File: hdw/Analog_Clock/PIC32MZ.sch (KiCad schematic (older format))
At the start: 3 parts

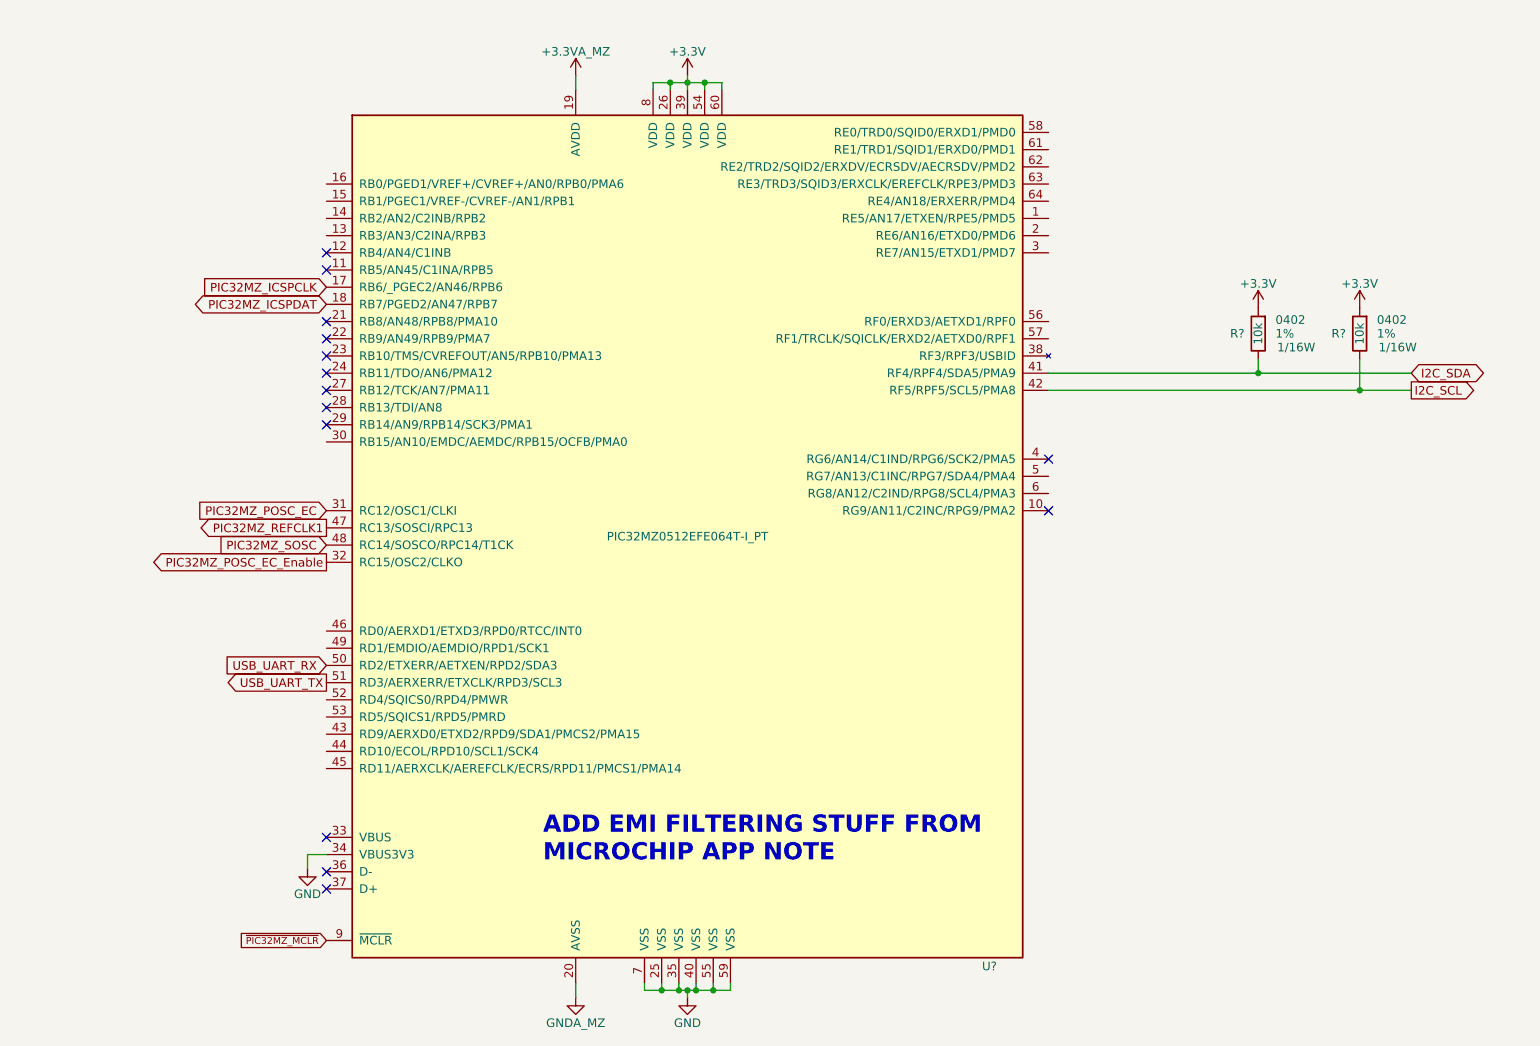
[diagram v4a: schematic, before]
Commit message: more analog work, added some more sch stuff
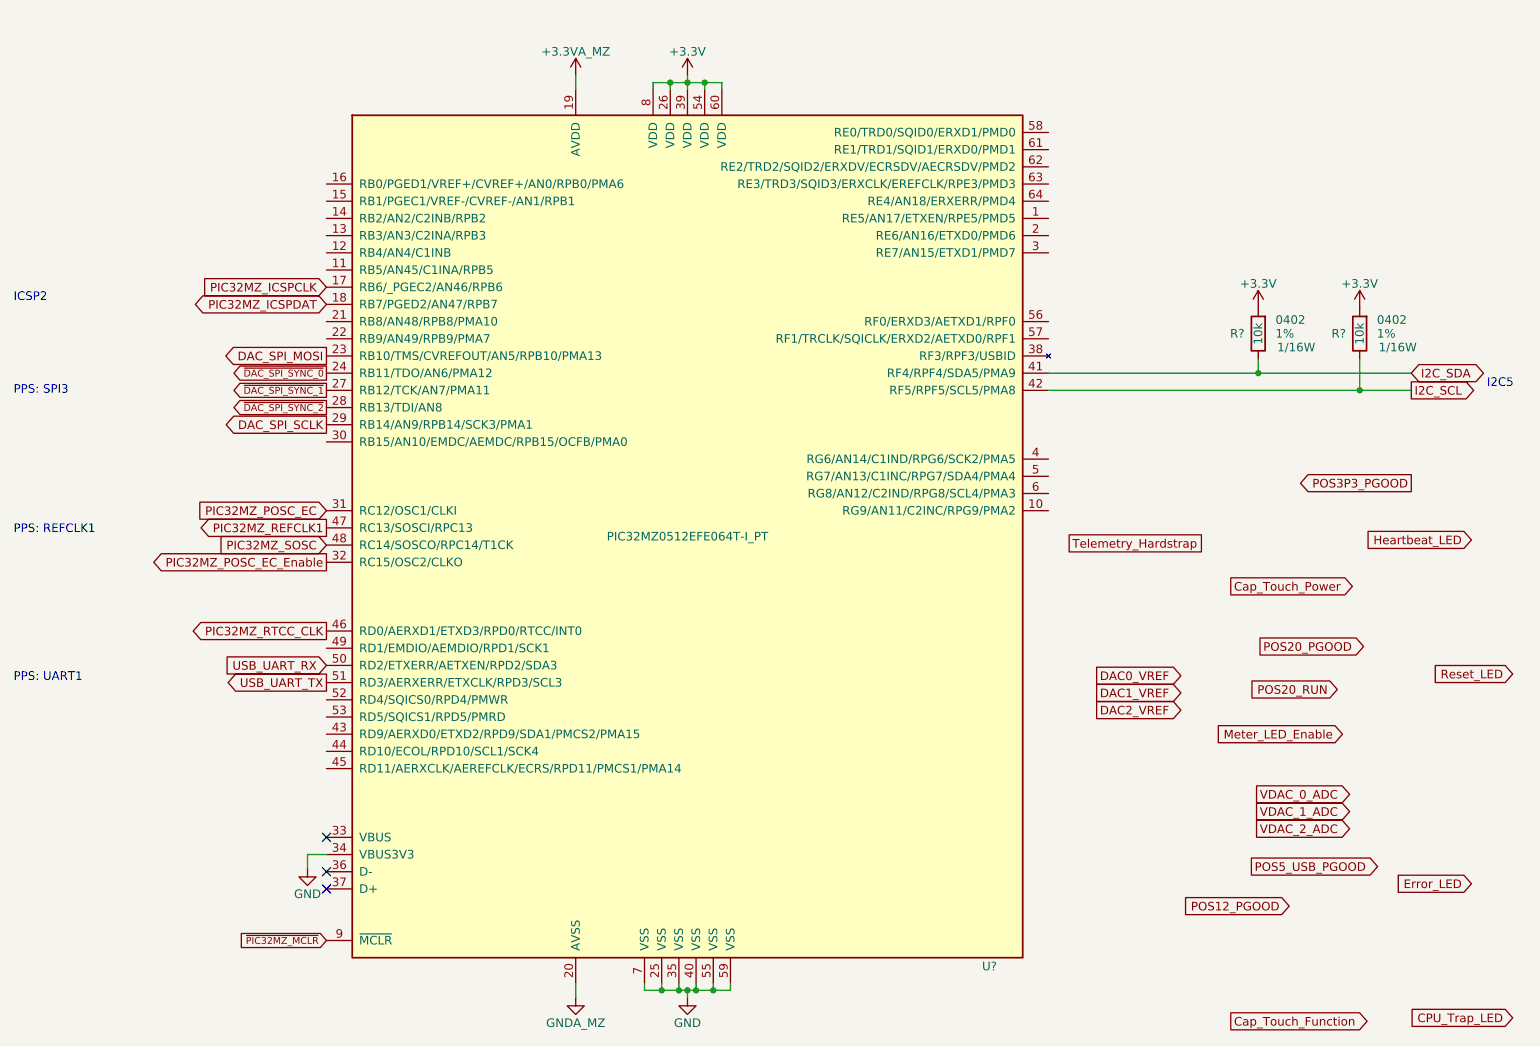
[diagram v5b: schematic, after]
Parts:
- removed U?: PIC32MZ0512EFE064T-I_PT, Package_QFP:TQFP-64_10x10mm_P0.5mm, symbol Custom_Library:PIC32MZ0512EFE064T-I_PT
- added U?: PIC32MZ0512EFE064T-I_PT, Package_QFP:TQFP-64_10x10mm_P0.5mm, symbol Custom_Library:PIC32MZ0512EFE064T-I_PT
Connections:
- net +3.3VA_MZ: now also U?.19 (AVDD)
- net +3V3: now also U?.26 (VDD), U?.39 (VDD), U?.54 (VDD), U?.60 (VDD), U?.8 (VDD)
- net GND: now also U?.25 (VSS), U?.34 (VBUS3V3), U?.35 (VSS), U?.40 (VSS), U?.55 (VSS), U?.59 (VSS), U?.7 (VSS)
- net GNDA_MZ: now also U?.20 (AVSS)
- net I2C_SCL: now also U?.42 (RF5/RPF5/SCL5/PMA8)
- net I2C_SDA: now also U?.41 (RF4/RPF4/SDA5/PMA9)
- net PIC32MZ_ICSPCLK: now also U?.17 (RB6/_PGEC2/AN46/RPB6)
- net PIC32MZ_ICSPDAT: now also U?.18 (RB7/PGED2/AN47/RPB7)
- net PIC32MZ_POSC_EC: now also U?.31 (RC12/OSC1/CLKI)
- net PIC32MZ_POSC_EC_Enable: now also U?.32 (RC15/OSC2/CLKO)
- net PIC32MZ_REFCLK1: now also U?.47 (RC13/SOSCI/RPC13)
- net PIC32MZ_SOSC: now also U?.48 (RC14/SOSCO/RPC14/T1CK)
- net USB_UART_RX: now also U?.50 (RD2/ETXERR/AETXEN/RPD2/SDA3)
- net USB_UART_TX: now also U?.51 (RD3/AERXERR/ETXCLK/RPD3/SCL3)
- net ~PIC32MZ_MCLR: now also U?.9 (~MCLR~)
- new net DAC_SPI_MOSI: U?.23 (RB10/TMS/CVREFOUT/AN5/RPB10/PMA13)
- new net DAC_SPI_SCLK: U?.29 (RB14/AN9/RPB14/SCK3/PMA1)
- new net PIC32MZ_RTCC_CLK: U?.46 (RD0/AERXD1/ETXD3/RPD0/RTCC/INT0)
- new net ~DAC_SPI_SYNC_0: U?.24 (RB11/TDO/AN6/PMA12)
- new net ~DAC_SPI_SYNC_1: U?.27 (RB12/TCK/AN7/PMA11)
- new net ~DAC_SPI_SYNC_2: U?.28 (RB13/TDI/AN8)
- no-connect marks 14 -> 3
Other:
- note added: "I2C5"
- note added: "ICSP2"
- note added: "PPS: REFCLK1"
- note added: "PPS: SPI3"
- note added: "PPS: UART1"
- note removed: "ADD EMI FILTERING STUFF FROM\nMICROCHIP APP NOTE"
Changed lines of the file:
@@
 $Descr A 11000 8500
 encoding utf-8
-Sheet 10 23
+Sheet 10 24
 Title "Pulse Oximeter"
 Date "2020-08-01"
@@
 NoConn ~ 3320 5680
 NoConn ~ 3320 5780
-$Comp
-L Custom_Library:PIC32MZ0512EFE064T-I_PT U?
-U 1 1 5EB2446C
-P 5420 3730
-F 0 "U?" H 7220 1230 50  0000 R CNN
-F 1 "PIC32MZ0512EFE064T-I_PT" H 5420 3730 50  0000 C CNN
-F 2 "Package_QFP:TQFP-64_10x10mm_P0.5mm" H 5420 3730 50  0001 C CNN
-F 3 "http://ww1.microchip.com/downloads/en/DeviceDoc/60001320E.pdf" H 5420 3730 50  0001 C CNN
-F 4 "PIC32MZ0512EFE064T-I/PTCT-ND" H 5420 3730 50  0001 C CNN "Digi-Key PN"
-	1    5420 3730
-	1    0    0    -1
-$EndComp
 Text GLabel 3320 3680 0    50   Output ~ 0
 PIC32MZ_REFCLK1
@@
 Wire Wire Line
 	9330 2880 9630 2880
-NoConn ~ 3320 2080
-NoConn ~ 3320 2180
-NoConn ~ 3320 2780
-NoConn ~ 3320 2880
-NoConn ~ 7520 3280
-NoConn ~ 7520 3580
-NoConn ~ 3320 2480
-NoConn ~ 3320 2580
-NoConn ~ 3320 2680
-NoConn ~ 3320 2980
-NoConn ~ 3320 3080
-Text Notes 4580 5630 0    100  ~ 20
-ADD EMI FILTERING STUFF FROM\nMICROCHIP APP NOTE
 Text GLabel 3320 3780 0    50   Input ~ 0
 PIC32MZ_SOSC
+$Comp
+L Custom_Library:PIC32MZ0512EFE064T-I_PT U?
+U 1 1 5F3A240D
+P 5420 3730
+F 0 "U?" H 7220 1230 50  0000 R CNN
+F 1 "PIC32MZ0512EFE064T-I_PT" H 5420 3730 50  0000 C CNN
+F 2 "Package_QFP:TQFP-64_10x10mm_P0.5mm" H 5420 3730 50  0001 C CNN
+F 3 "http://ww1.microchip.com/downloads/en/DeviceDoc/60001320E.pdf" H 5420 3730 50  0001 C CNN
+F 4 "PIC32MZ0512EFE064T-I/PTCT-ND" H 5420 3730 50  0001 C CNN "Digi-Key PN"
+	1    5420 3730
+	1    0    0    -1
+$EndComp
+Text Notes 10070 2870 0    50   ~ 0
+I2C5
+Text Notes 1500 4580 0    50   ~ 0
+PPS: UART1
+Text Notes 1500 3720 0    50   ~ 0
+PPS: REFCLK1
+Text GLabel 3320 2680 0    50   Output ~ 0
+DAC_SPI_MOSI
+Text GLabel 3320 3080 0    50   Output ~ 0
+DAC_SPI_SCLK
+Text GLabel 3320 2780 0    40   Output ~ 0
+~DAC_SPI_SYNC_0
+Text GLabel 3320 2880 0    40   Output ~ 0
+~DAC_SPI_SYNC_1
+Text GLabel 3320 2980 0    40   Output ~ 0
+~DAC_SPI_SYNC_2
+Text Notes 1500 2910 0    50   ~ 0
+PPS: SPI3
+Text GLabel 8730 5230 2    50   Output ~ 0
+VDAC_0_ADC
+Text GLabel 8730 5330 2    50   Output ~ 0
+VDAC_1_ADC
+Text GLabel 8730 5430 2    50   Output ~ 0
+VDAC_2_ADC
+Text Notes 1500 2370 0    50   ~ 0
+ICSP2
+Text GLabel 3320 4280 0    50   Output ~ 0
+PIC32MZ_RTCC_CLK
+Text GLabel 9230 4880 0    50   Input ~ 0
+Meter_LED_Enable
+Text GLabel 8580 4020 2    50   Output ~ 0
+Cap_Touch_Power
+Text GLabel 8580 6550 2    50   Output ~ 0
+Cap_Touch_Function
+Text GLabel 9200 4620 0    50   Input ~ 0
+POS20_RUN
+Text GLabel 8750 4370 2    50   Output ~ 0
+POS20_PGOOD
+Text GLabel 8920 5880 0    50   Input ~ 0
+POS12_PGOOD
+Text GLabel 9630 3420 0    50   Output ~ 0
+POS3P3_PGOOD
+Text GLabel 8700 5650 2    50   Output ~ 0
+POS5_USB_PGOOD
+Text GLabel 9980 3750 0    50   Input ~ 0
+Heartbeat_LED
+Text GLabel 9980 5750 0    50   Input ~ 0
+Error_LED
+Text GLabel 10220 4530 0    50   Input ~ 0
+Reset_LED
+Text GLabel 10220 6530 0    50   Input ~ 0
+CPU_Trap_LED
+Text GLabel 7800 4540 2    50   Output ~ 0
+DAC0_VREF
+Text GLabel 7800 4640 2    50   Output ~ 0
+DAC1_VREF
+Text GLabel 7800 4740 2    50   Output ~ 0
+DAC2_VREF
+Text GLabel 7640 3770 2    50   UnSpc ~ 0
+Telemetry_Hardstrap
 $EndSCHEMATC
